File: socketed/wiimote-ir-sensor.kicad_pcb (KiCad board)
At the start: 2 copper layers, 13.5 x 16.2 mm, 10 parts, among them J1 Conn_01x04_Pin, U2 AP2112-3.3V, X1 SG3225CAN 24.0000M-TJGA3

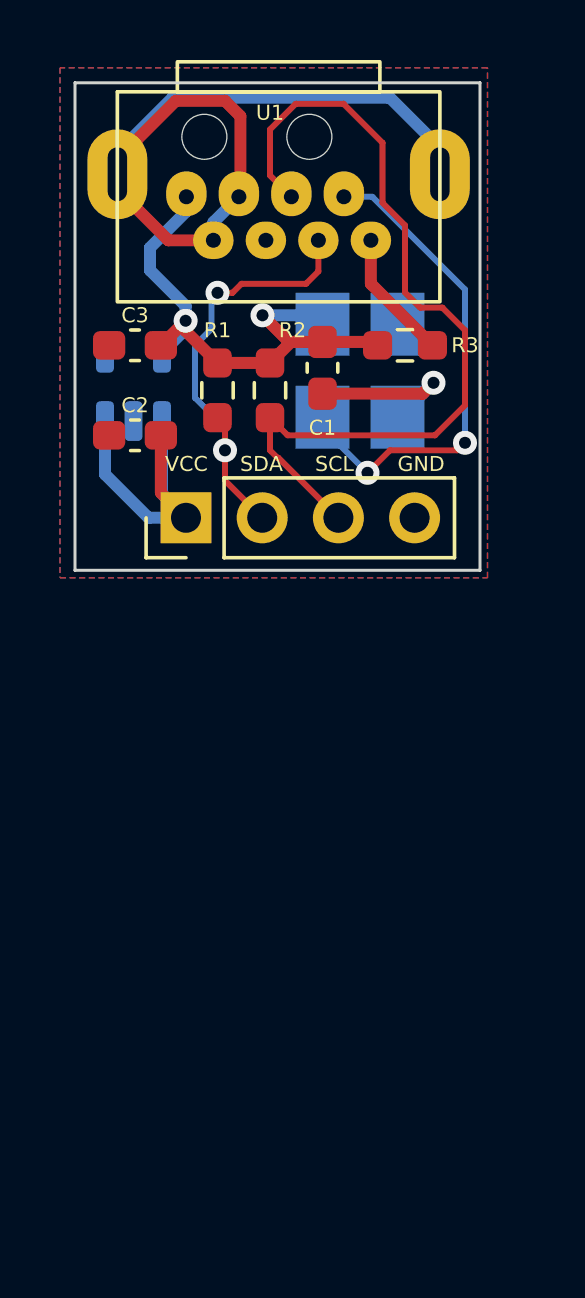
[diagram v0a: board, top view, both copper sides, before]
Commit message: Socketed board: Tidy up
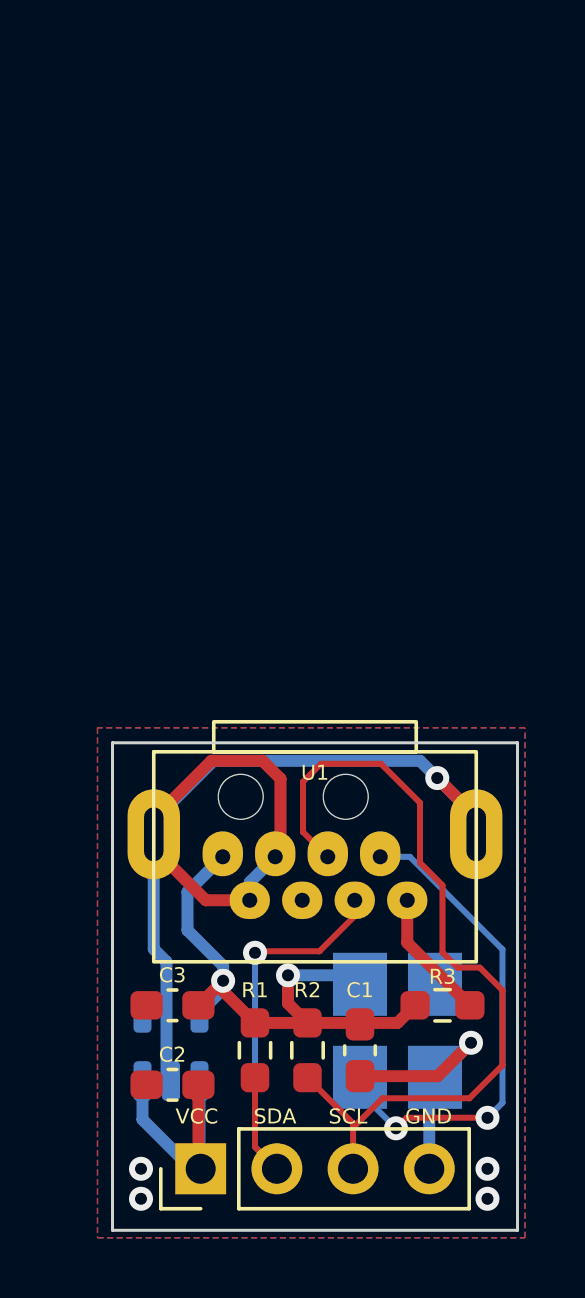
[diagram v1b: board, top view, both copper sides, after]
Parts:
- moved C1 22.8 mm to (158.2, 110.2)
- moved U1 22.0 mm to (156.8, 102.8)
- moved C3 22.0 mm to (152.0, 108.8)
- moved R1 22.0 mm to (154.8, 110.2)
- moved R2 22.0 mm to (156.5, 110.2)
- moved R3 22.0 mm to (161.0, 108.8)
- moved U2 22.0 mm to (151.9, 110.1)
- moved X1 22.0 mm to (159.5, 109.6)
- moved J1 21.7 mm to (152.9, 114.2)
- moved C2 21.7 mm to (152.0, 111.4)
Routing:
- net GND: track 30.5 -> 44.8 mm, vias 1 -> 6
- net +5V: track 11.7 -> 10.2 mm
- net /SCL: track 29.0 -> 27.7 mm
- net /CLK: track 17.2 -> 16.6 mm
- net /SDA: track 14.3 -> 14.7 mm, vias 2 -> 1

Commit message: More QoL tweaks to socketed board
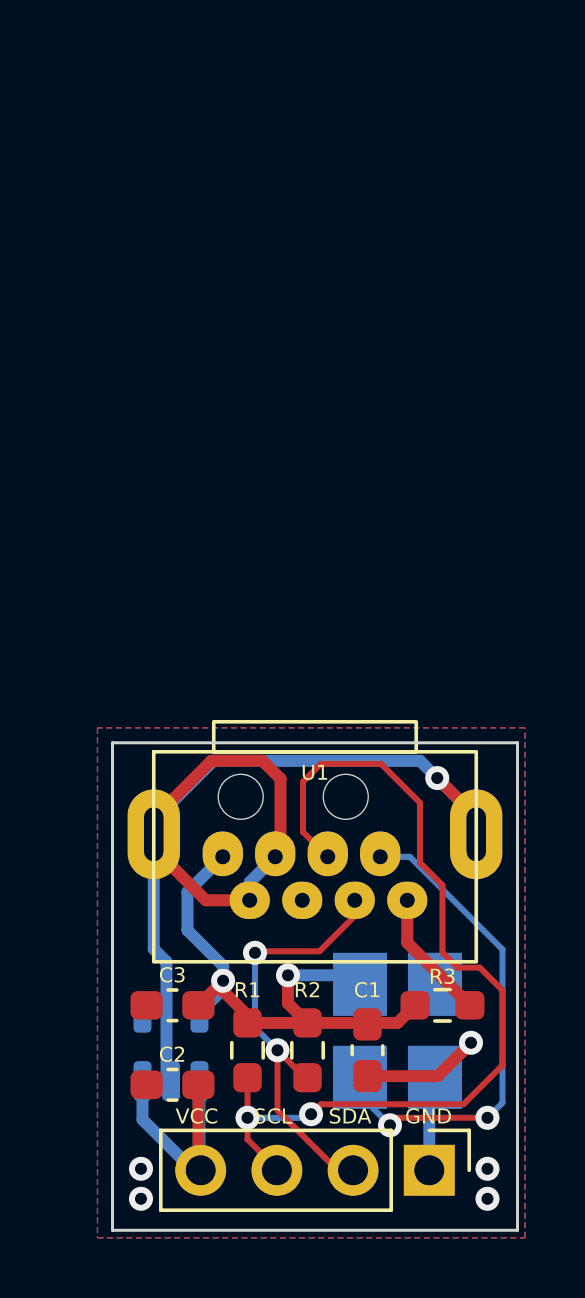
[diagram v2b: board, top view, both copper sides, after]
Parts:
- R3: value 330K -> 33K
- moved J1 7.62 mm to (160.6, 114.2), turned to -90 degrees
- moved C1 0.25 mm to (158.5, 110.2)
- moved R1 0.25 mm to (154.5, 110.2)
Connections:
- J1 pad 1: +5V -> GND
- J1 pad 4: GND -> +5V
- R1 pad 2: /SDA -> /SCL
- R2 pad 1: /SCL -> /SDA
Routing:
- net /SCL: track 27.7 -> 30.5 mm, vias 0 -> 2
- net /SDA: track 14.7 -> 13.4 mm, vias 1 -> 2
- net GND: track 44.8 -> 43.9 mm
